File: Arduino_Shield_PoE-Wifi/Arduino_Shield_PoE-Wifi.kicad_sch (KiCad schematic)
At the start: 11 parts, among them J1 Conn_02x08, J2 Conn_02x08, J3 PINHD_1x2_Female, J4 PINHD_1x2_Female, SW1 Push_Button

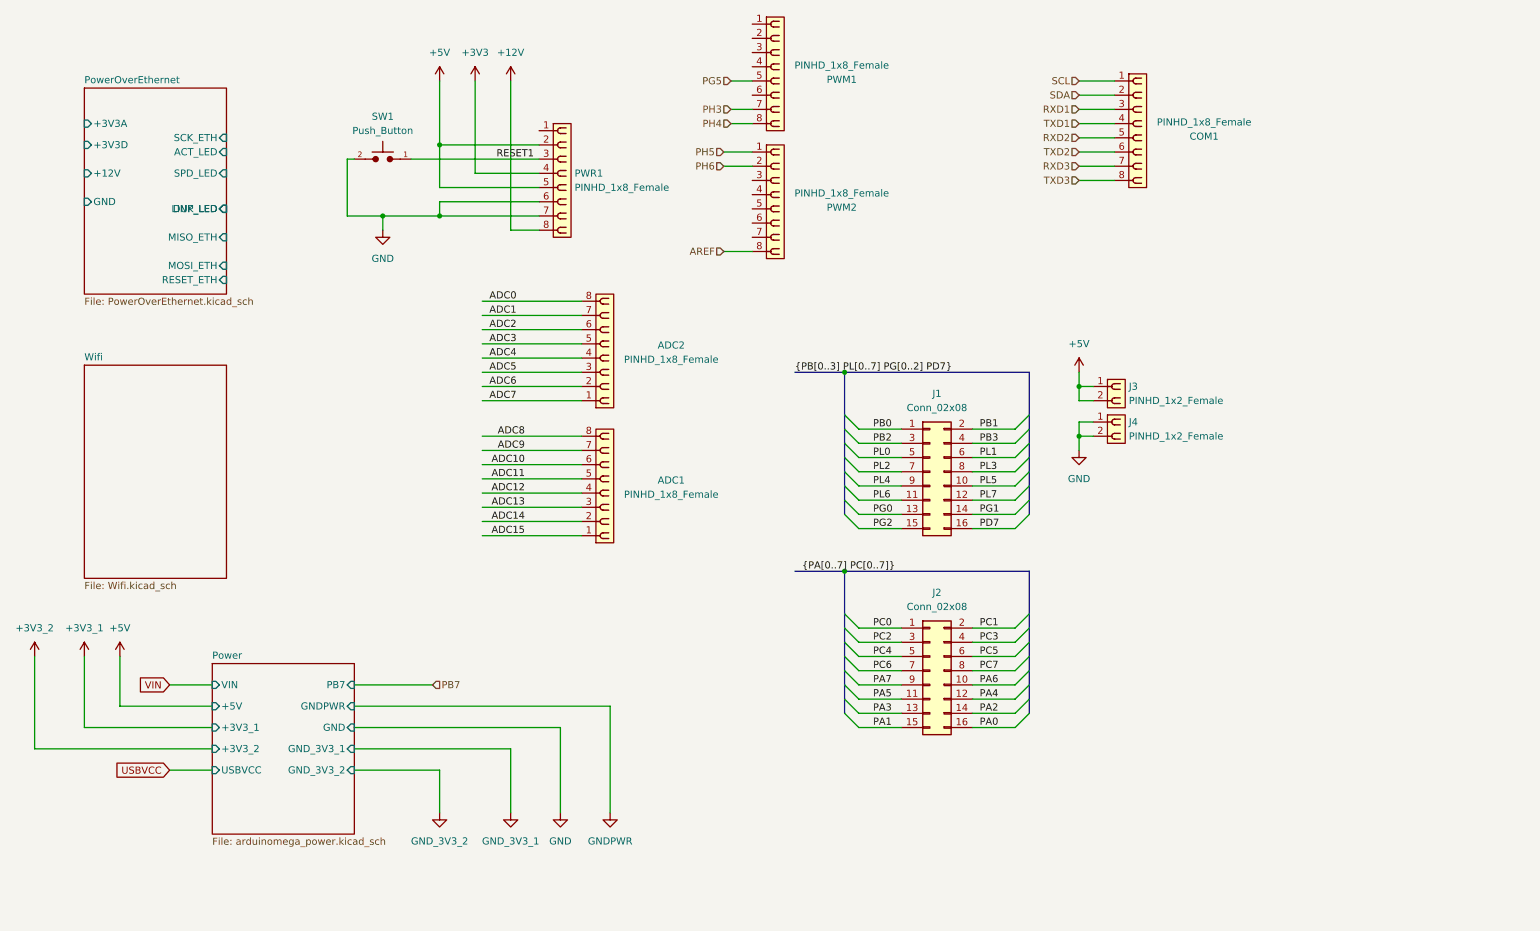
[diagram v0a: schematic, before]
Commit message: Update
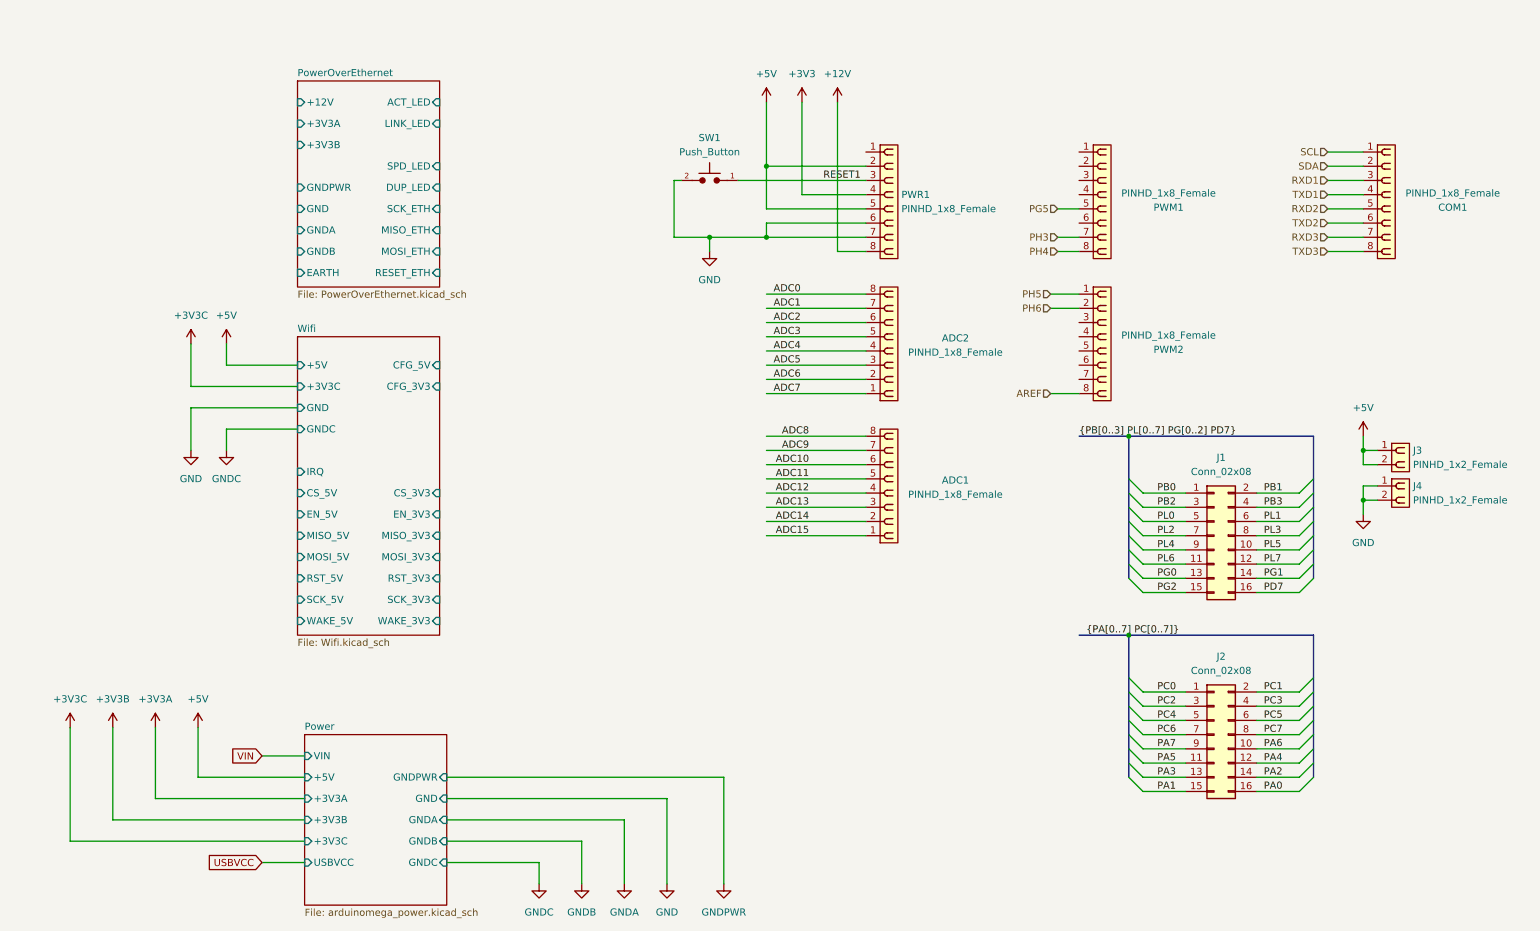
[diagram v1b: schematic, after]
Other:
- sheet Power ports: added +3V3A, +3V3B, +3V3C, GNDA, GNDB, GNDC; removed +3V3_1, +3V3_2, GND_3V3_1, GND_3V3_2, PB7
- sheet PowerOverEthernet ports: added +3V3B, EARTH, GNDA, GNDB, GNDPWR; removed +3V3D
- sheet Wifi ports: added +3V3C, +5V, CFG_3V3, CFG_5V, CS_3V3, CS_5V, EN_3V3, EN_5V, GND, GNDC, IRQ, MISO_3V3, MISO_5V, MOSI_3V3, MOSI_5V, RST_3V3, RST_5V, SCK_3V3, SCK_5V, WAKE_3V3, WAKE_5V; removed none
- moved on the sheet: ADC1, ADC2, COM1, J1, J2, J3, J4, PWM1, PWM2, PWR1, SW1
